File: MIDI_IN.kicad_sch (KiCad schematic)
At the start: 5 parts, among them IC201 TLP293_GR-TPL,E, J201 DIN-5_180degree

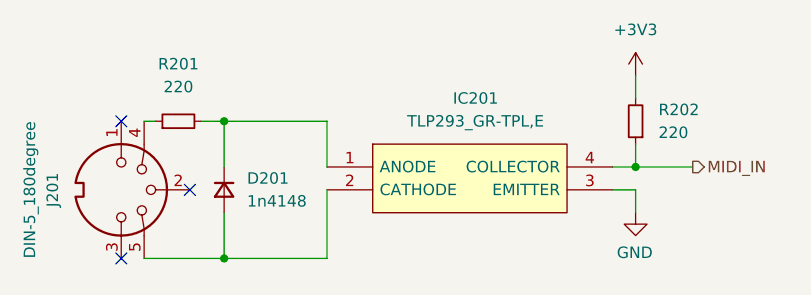
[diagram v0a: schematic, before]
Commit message: Finish IO design
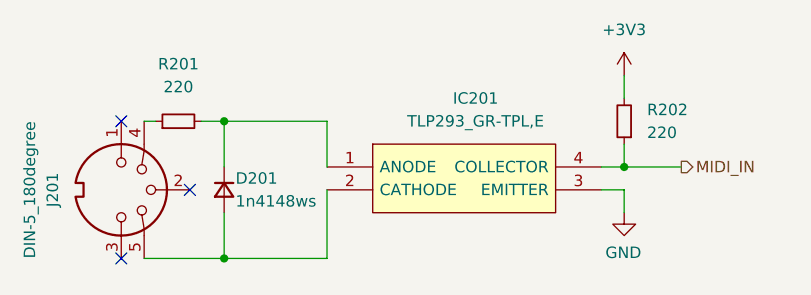
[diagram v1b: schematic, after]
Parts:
- D201: value 1n4148 -> 1n4148ws; footprint (none) -> Diode_SMD:D_SOD-323
- IC201: footprint (none) -> Footprints:SOIC127P700X230-4N
- R201, R202: footprint (none) -> Resistor_SMD:R_0603_1608Metric_Pad0.98x0.95mm_HandSolder
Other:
- moved on the sheet: IC201, R202
